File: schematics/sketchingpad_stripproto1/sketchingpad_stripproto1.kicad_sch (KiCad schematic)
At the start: 83 parts, among them CN1 HC-1.0-4PWT, CN2 S2B-PH-SM4-TB, J3 AudioJack4, Q1 AO3415A, SW1 TC-S3601-3.5-260G-F0.6, SW2 MINI MSK12CO2, U1 TS20, U2 Seeeduino Xiao nRF52840

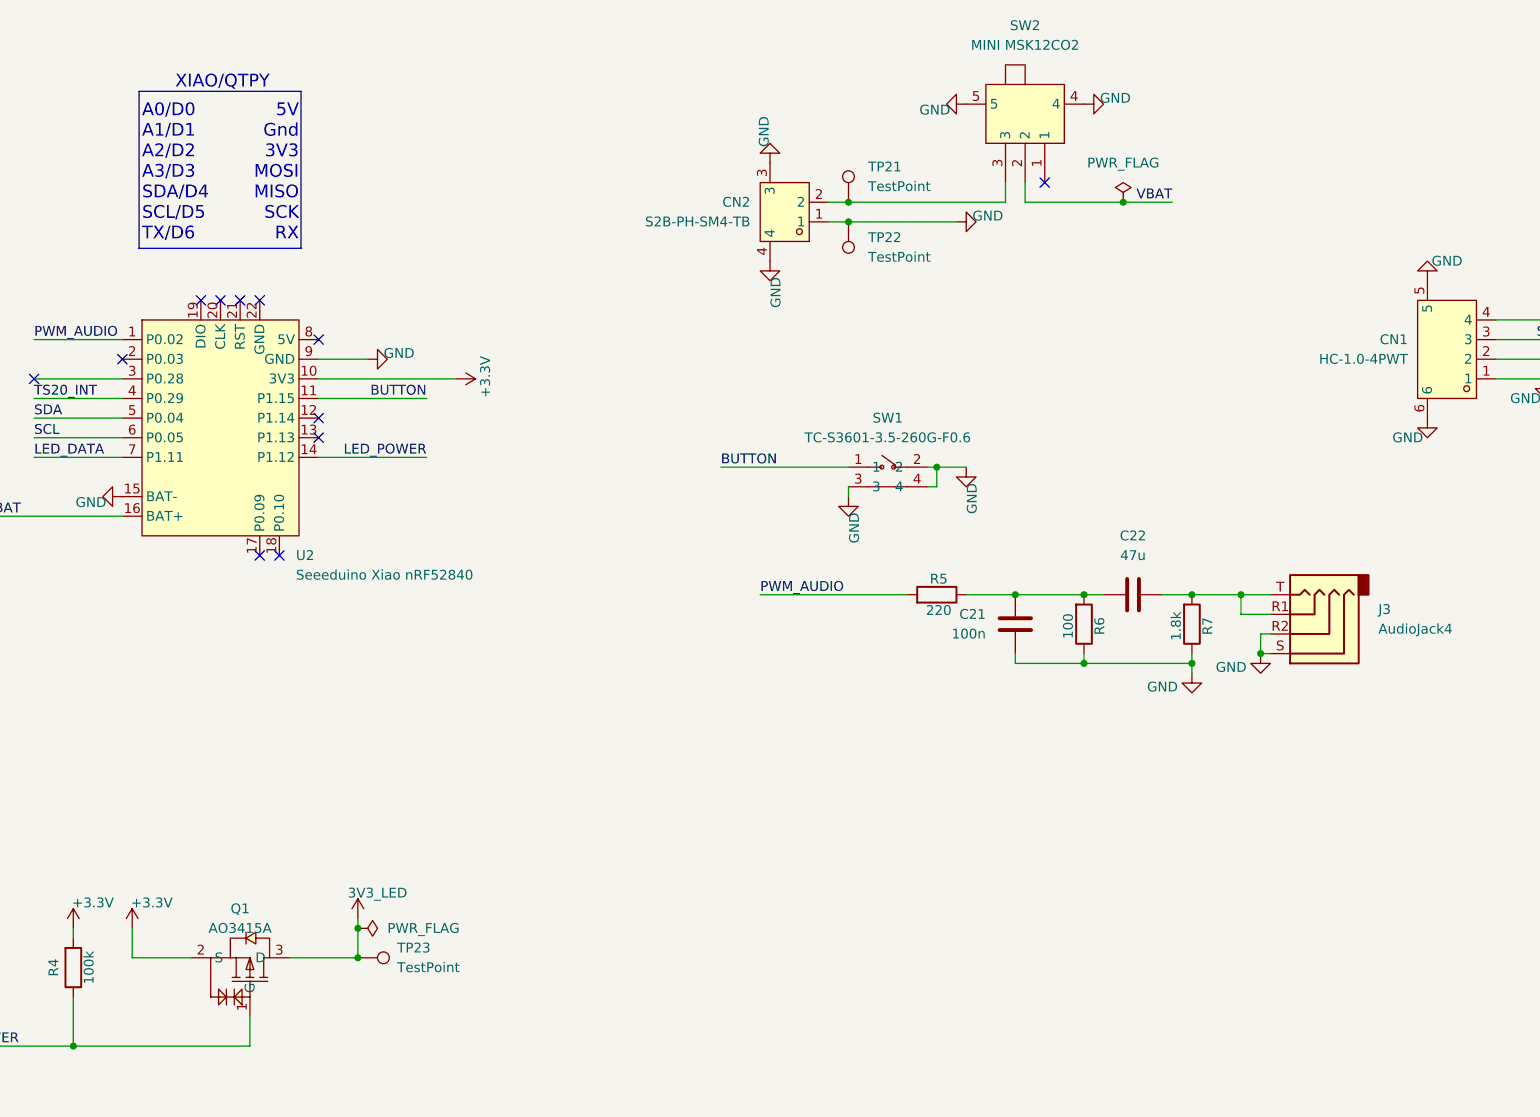
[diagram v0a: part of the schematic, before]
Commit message: ERC and DRC pass
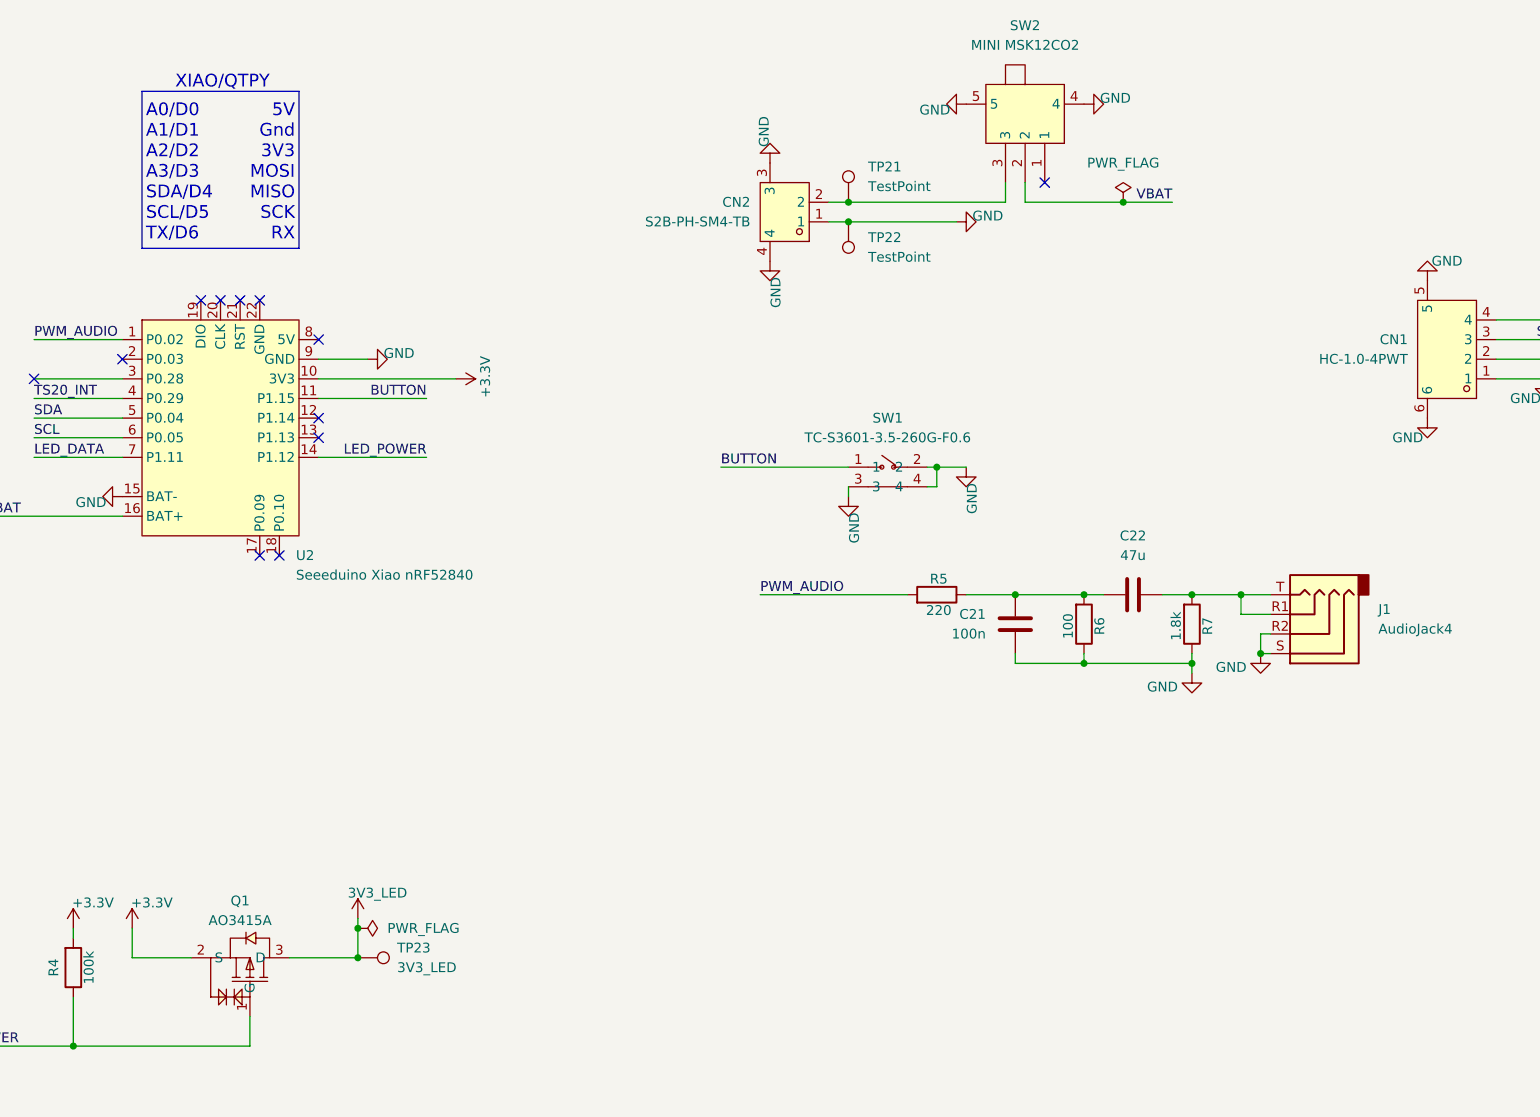
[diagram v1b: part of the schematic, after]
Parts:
- TP23: value TestPoint -> 3V3_LED
- renumbered J3 to J1
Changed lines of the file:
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@@
 	(paper "A3")
 	(rectangle
-		(start 47.879 22.479)
-		(end 68.834 42.799)
+		(start 48.26 22.479)
+		(end 68.58 42.799)
 		(stroke
 			(width 0)
@@
 	(text "A0/D0\nA1/D1\nA2/D2\nA3/D3\nSDA/D4\nSCL/D5\nTX/D6"
 		(exclude_from_sim no)
-		(at 48.26 33.02 0)
+		(at 48.768 33.02 0)
 		(effects
 			(font
@@
 	(text "5V\nGnd\n3V3\nMOSI\nMISO\nSCK\nRX"
 		(exclude_from_sim no)
-		(at 68.58 33.02 0)
+		(at 68.072 33.02 0)
 		(effects
 			(font
@@
 		(dnp no)
 		(fields_autoplaced yes)
-		(property "Reference" "J3"
+		(property "Reference" "J1"
 			(at 208.28 89.5349 0)
 			(show_name no)
@@
 			)
 		)
+		(property "DigikeyPN" ""
+			(at 199.39 92.71 0)
+			(hide yes)
+			(show_name no)
+			(do_not_autoplace no)
+			(effects
+				(font
+					(size 1.27 1.27)
+				)
+			)
+		)
+		(property "MPN" ""
+			(at 199.39 92.71 0)
+			(hide yes)
+			(show_name no)
+			(do_not_autoplace no)
+			(effects
+				(font
+					(size 1.27 1.27)
+				)
+			)
+		)
+		(property "Note" ""
+			(at 199.39 92.71 0)
+			(show_name no)
+			(do_not_autoplace no)
+			(effects
+				(font
+					(size 1.27 1.27)
+				)
+			)
+		)
 		(pin "S"
 		)
@@
 			(project "sketchingpad_stripproto1"
 				(path "/69aff514-3aa6-493d-bc6d-4103dc0ce10d"
-					(reference "J3")
+					(reference "J1")
 					(unit 1)
 				)
@@
 			)
 		)
-		(property "Value" "TestPoint"
+		(property "Value" "3V3_LED"
 			(at 81.28 135.8899 90)
 			(show_name no)
@@
 		(in_pos_files yes)
 		(dnp no)
-		(fields_autoplaced yes)
 		(property "Reference" "Q1"
-			(at 60.96 128.27 90)
+			(at 60.96 127.254 90)
 			(show_name no)
 			(do_not_autoplace no)
@@
 		)
 		(property "Value" "AO3415A"
-			(at 60.96 130.81 90)
+			(at 60.96 129.794 90)
 			(show_name no)
 			(do_not_autoplace no)
@@
 			(show_name no)
 			(do_not_autoplace no)
+			(effects
+				(font
+					(size 1.27 1.27)
+				)
+			)
+		)
+		(property "DigikeyPN" ""
+			(at 133.35 38.1 0)
+			(hide yes)
+			(show_name no)
+			(do_not_autoplace no)
+			(effects
+				(font
+					(size 1.27 1.27)
+				)
+			)
+		)
+		(property "Note" ""
+			(at 133.35 38.1 0)
+			(show_name no)
+			(do_not_autoplace no)
